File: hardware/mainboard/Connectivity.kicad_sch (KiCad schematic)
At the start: 25 parts, among them U2 FT230XS

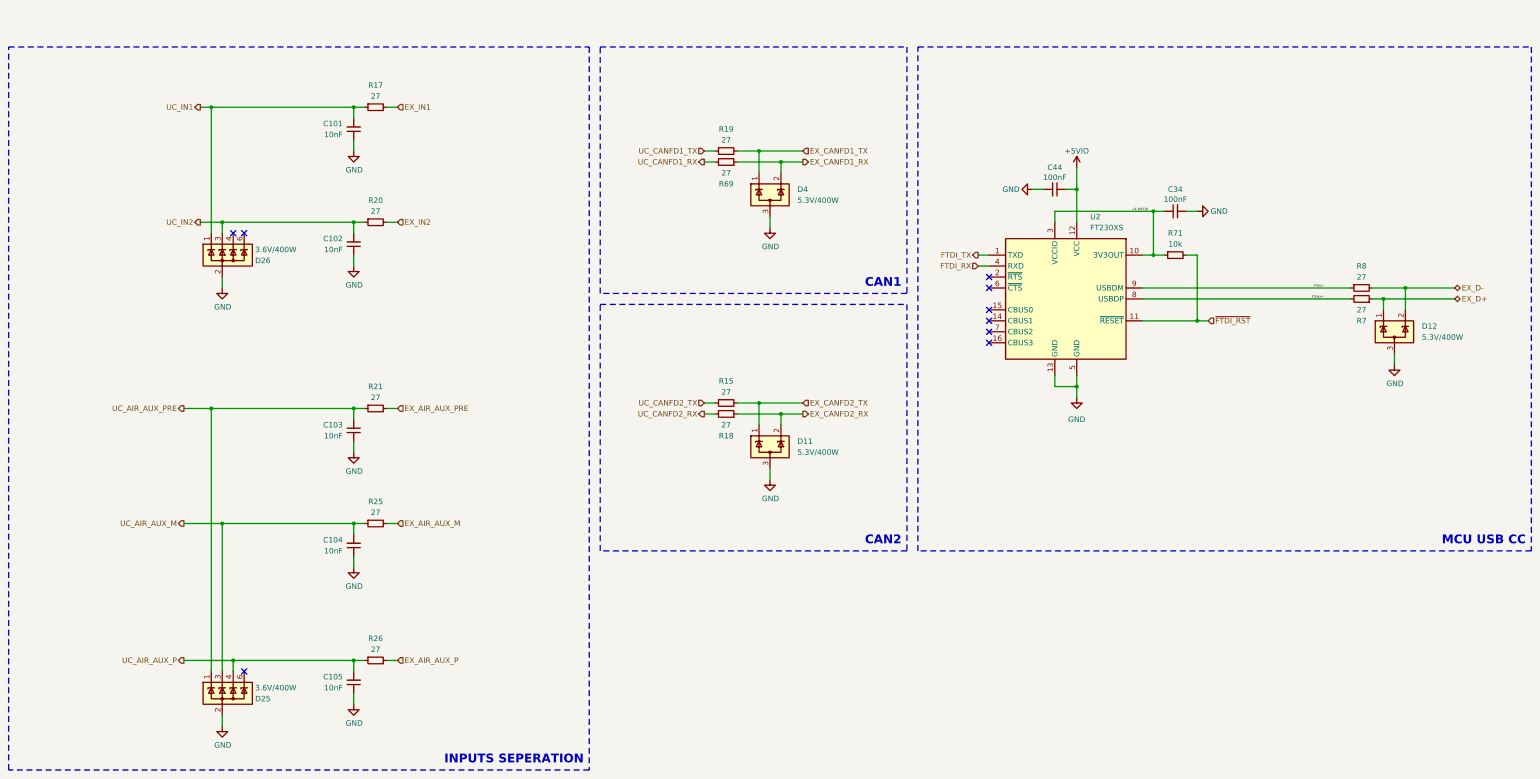
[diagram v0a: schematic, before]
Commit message: chore: sync
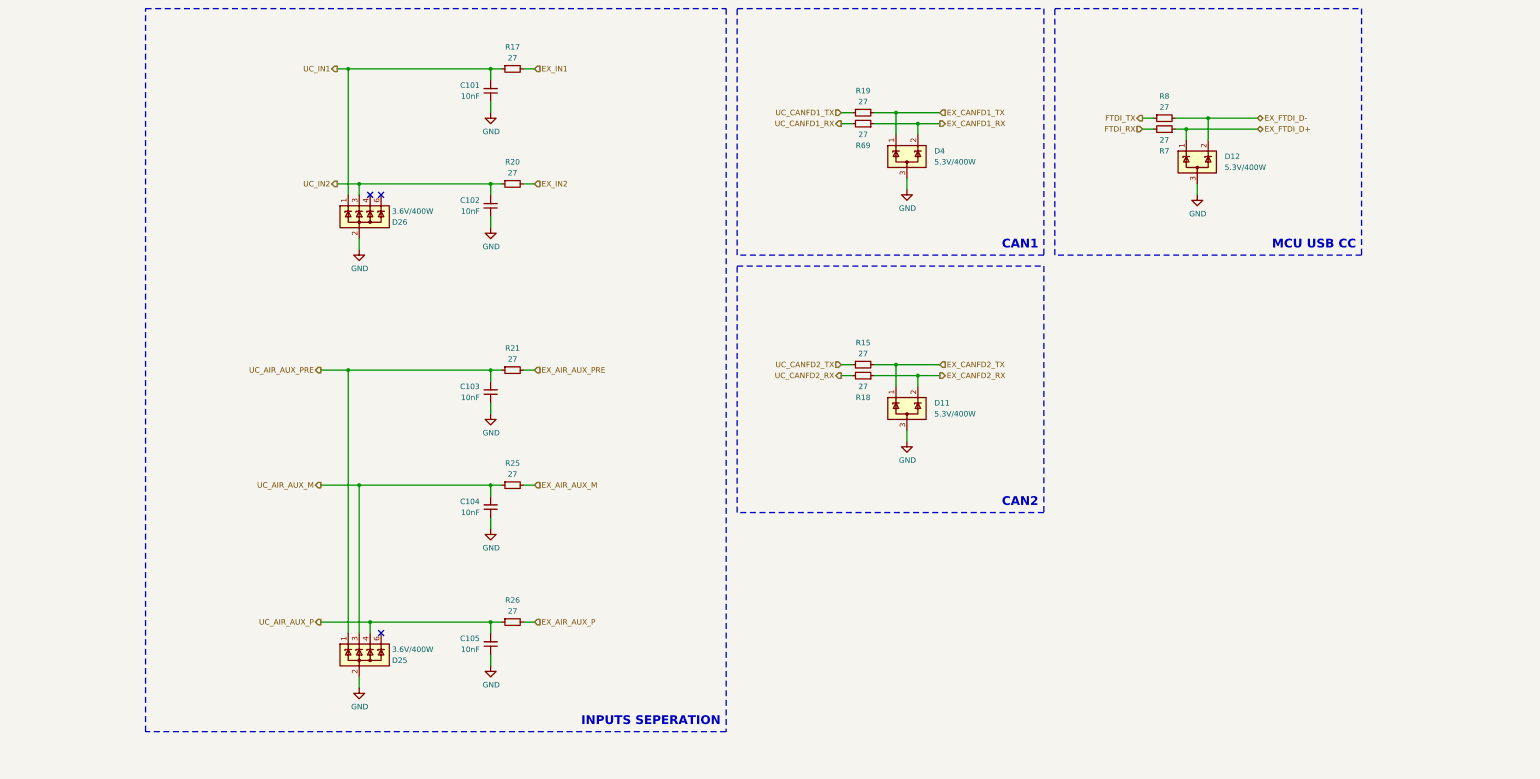
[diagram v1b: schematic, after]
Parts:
- removed C34, C44: 100nF, Capacitor_SMD:C_0603_1608Metric, symbol Device:C_Small
- removed R71: 10k, Resistor_SMD:R_0603_1608Metric, symbol Device:R_Small
- removed U2: FT230XS, Package_SO:SSOP-16_3.9x4.9mm_P0.635mm, symbol Interface_USB:FT230XS
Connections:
- net FTDIU+ is gone; now on net FTDI_RX: R7.2
- net FTDIU- is gone; now on net FTDI_TX: R8.1
- net EX_D+ renamed EX_FTDI_D+
- net EX_D- renamed EX_FTDI_D-
- no-connect marks 9 -> 3
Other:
- moved on the sheet: C101, C102, C103, C104, C105, D11, D12, D25, D26, D4, R15, R17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

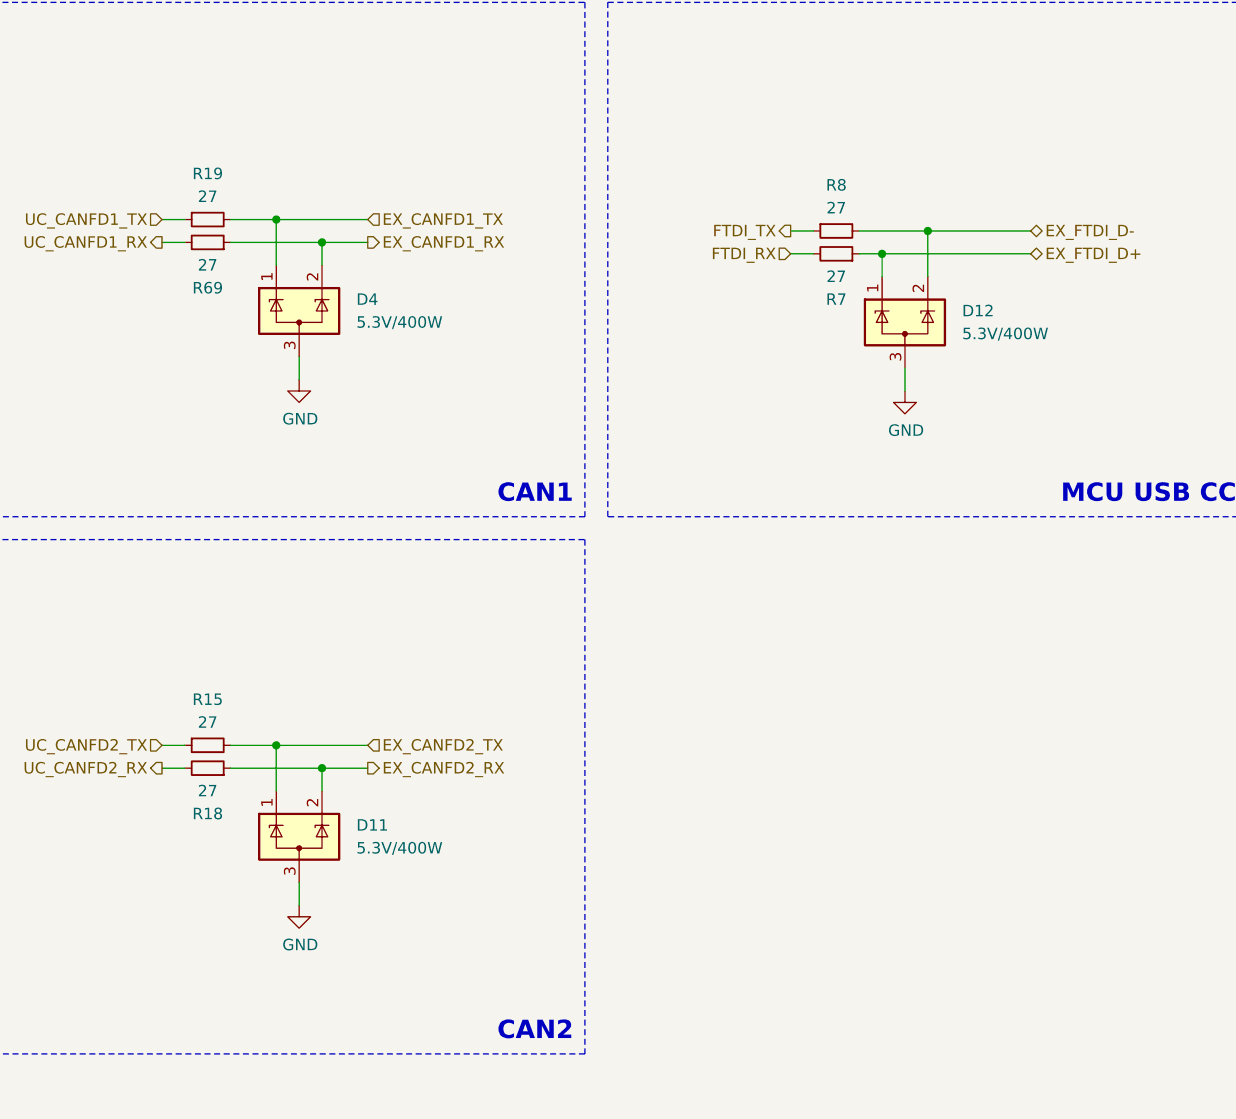
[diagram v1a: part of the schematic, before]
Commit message: chore: sync
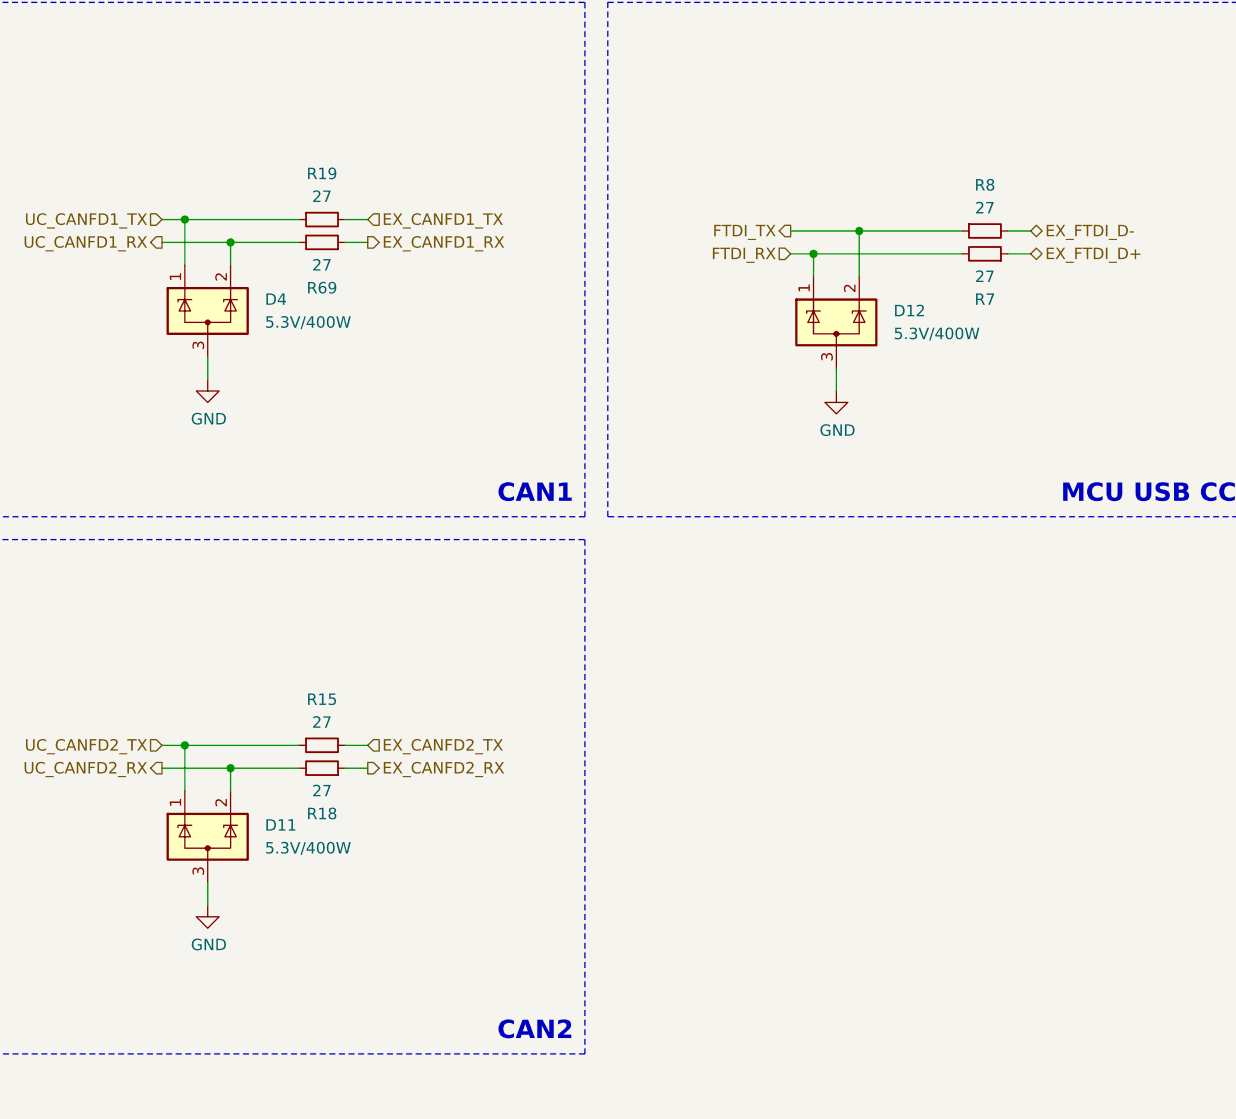
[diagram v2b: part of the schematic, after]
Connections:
- net EX_CANFD1_RX: no longer D4.2 (K)
- net EX_CANFD1_TX: no longer D4.1 (K)
- net EX_CANFD2_RX: no longer D11.2 (K)
- net EX_CANFD2_TX: no longer D11.1 (K)
- net EX_FTDI_D+: no longer D12.1 (K)
- net EX_FTDI_D-: no longer D12.2 (K)
- net FTDI_RX: now also D12.1 (K)
- net FTDI_TX: now also D12.2 (K)
- net UC_CANFD1_RX: now also D4.2 (K)
- net UC_CANFD1_TX: now also D4.1 (K)
- net UC_CANFD2_RX: now also D11.2 (K)
- net UC_CANFD2_TX: now also D11.1 (K)
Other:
- moved on the sheet: D11, D12, D4, R15, R18, R19, R69, R7, R8
